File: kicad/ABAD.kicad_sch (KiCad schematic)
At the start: 5 parts, among them U1 MS5611-01BA, U2 ESP32-WROOM-32, U3 MPU-6050

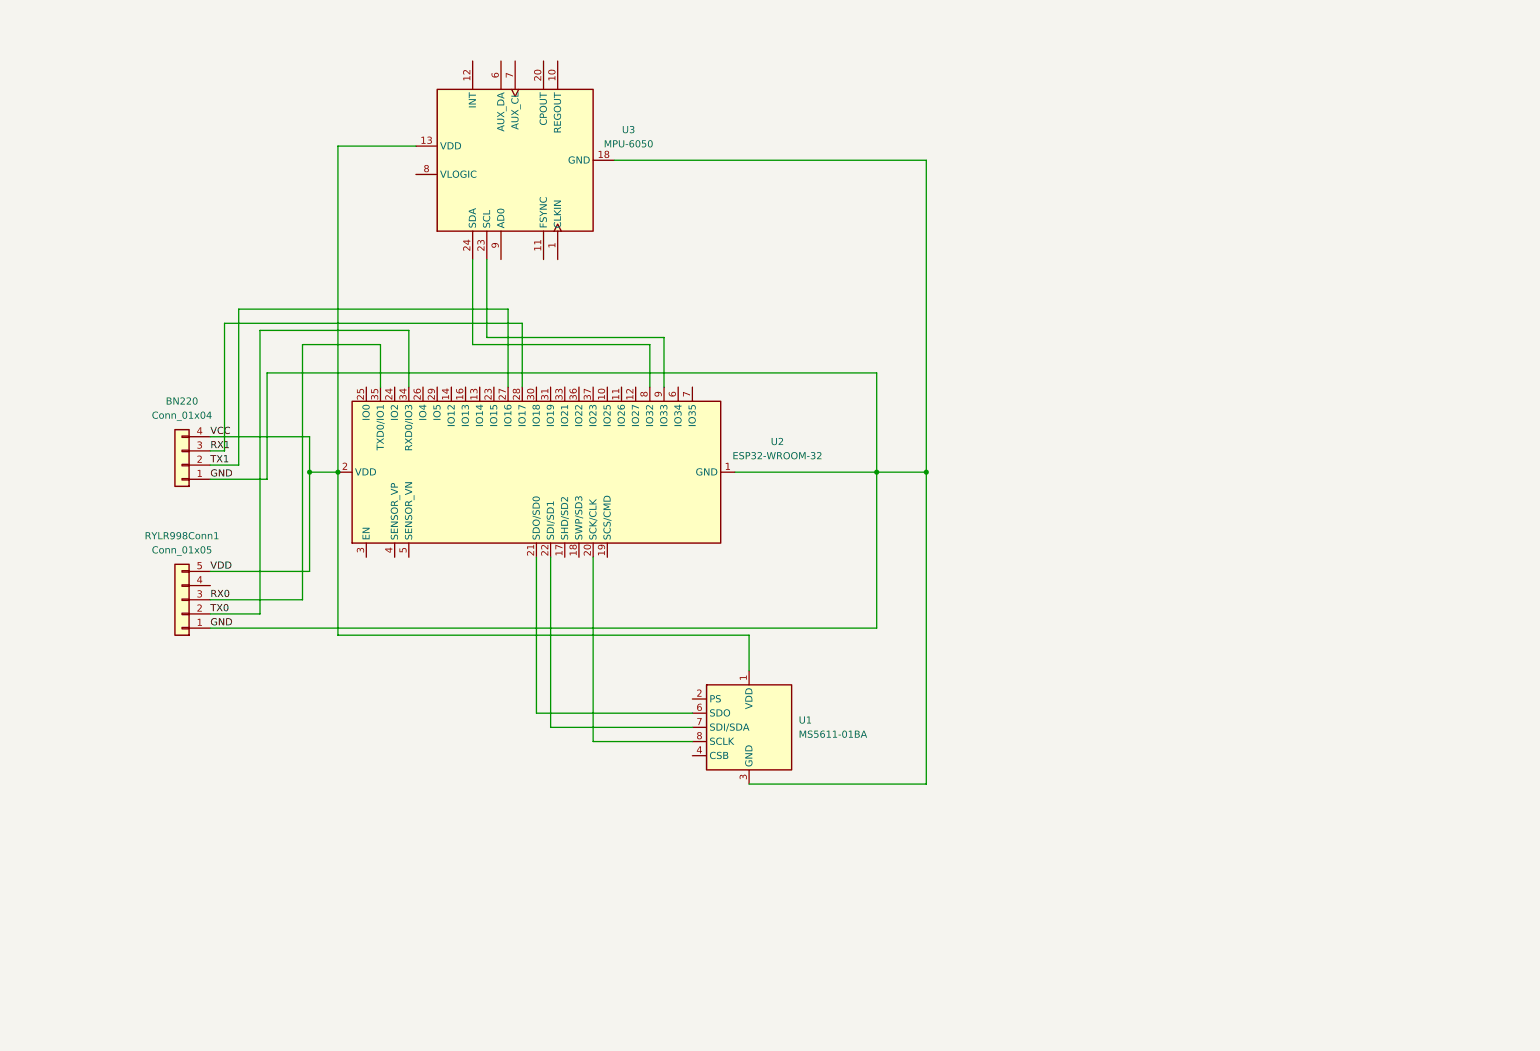
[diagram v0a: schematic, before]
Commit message: Schematic_Jul12_Nile
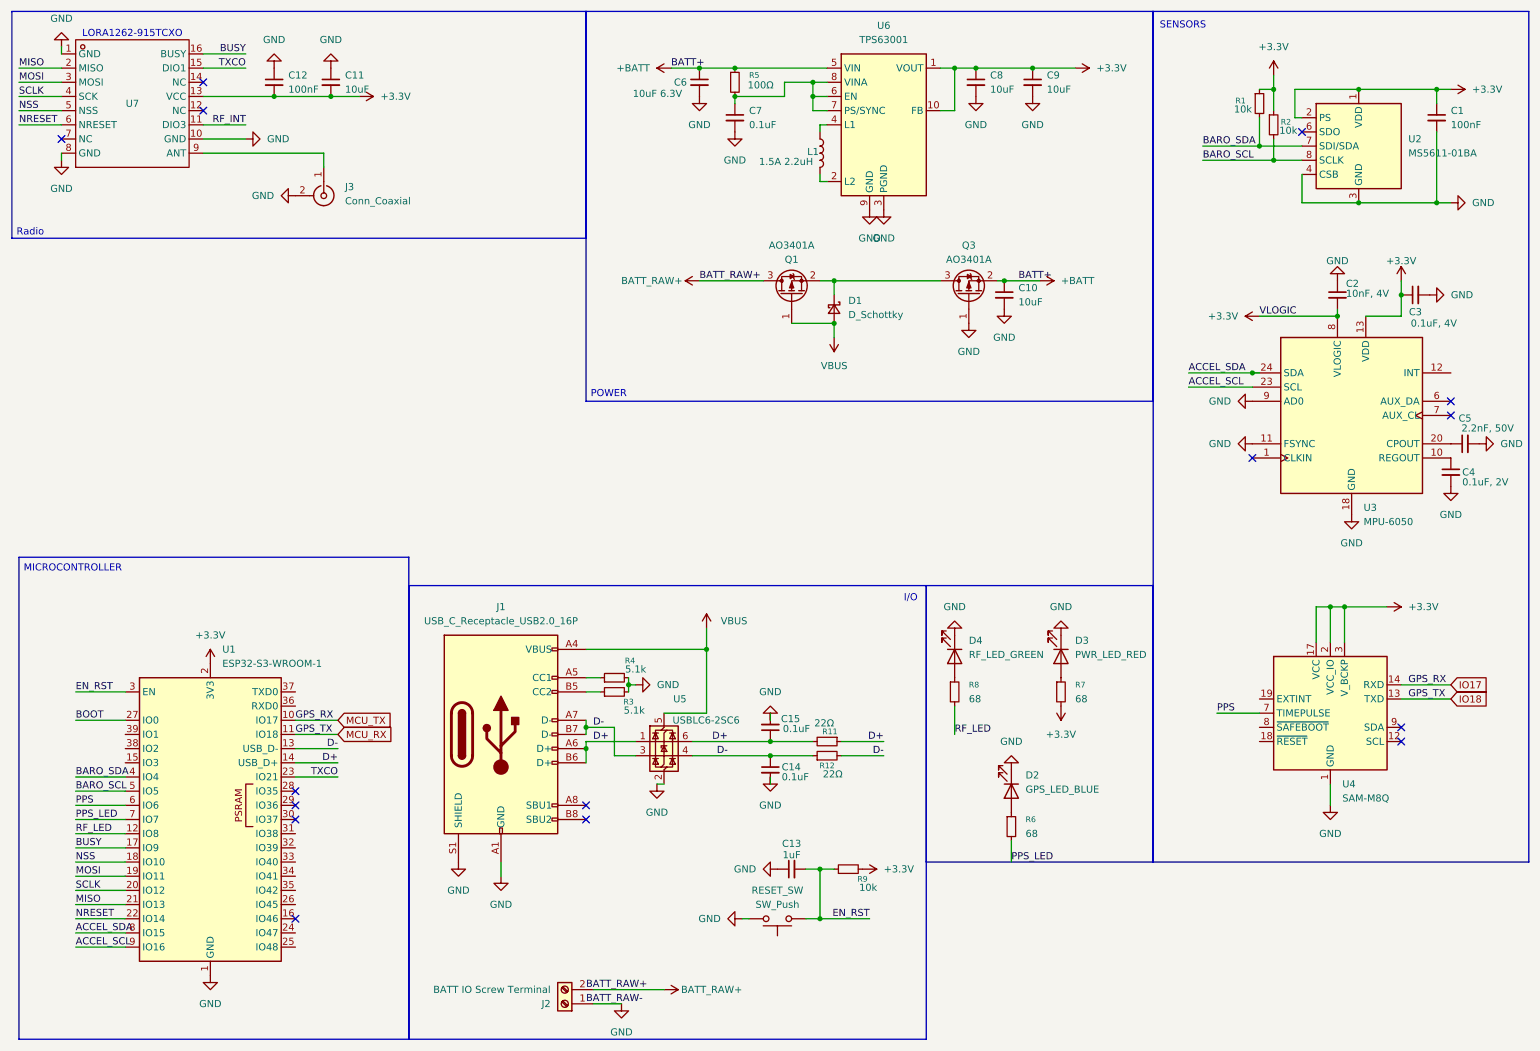
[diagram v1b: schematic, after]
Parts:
- removed BN220: Conn_01x04, Connector_JST:JST_SH_BM04B-SRSS-TB_1x04-1MP_P1.00mm_Vertical, symbol Connector_Generic:Conn_01x04
- removed RYLR998Conn1: Conn_01x05, Connector_PinSocket_1.00mm:PinSocket_1x05_P1.00mm_Vertical, symbol Connector_Generic:Conn_01x05
- removed U1: MS5611-01BA, Package_LGA:LGA-8_3x5mm_P1.25mm, symbol Sensor_Pressure:MS5611-01BA
- removed U2: ESP32-WROOM-32, RF_Module:ESP32-WROOM-32, symbol RF_Module:ESP32-WROOM-32
- added C1, C12: 100nF, Capacitor_SMD:C_0805_2012Metric, symbol Device:C_Small
- added C10, C11, C8, C9: 10uF, Capacitor_SMD:C_0805_2012Metric, symbol Device:C_Small
- added C13: 1uF, Capacitor_SMD:C_0805_2012Metric, symbol Device:C_Small
- added C14, C15, C7: 0.1uF, Capacitor_SMD:C_0805_2012Metric, symbol Device:C_Small
- added C2: 10nF, 4V, Capacitor_SMD:C_0805_2012Metric, symbol Device:C_Small
- added C3: 0.1uF, 4V, Capacitor_SMD:C_0805_2012Metric, symbol Device:C_Small
- added C4: 0.1uF, 2V, Capacitor_SMD:C_0805_2012Metric, symbol Device:C_Small
- added C5: 2.2nF, 50V, Capacitor_SMD:C_0805_2012Metric, symbol Device:C_Small
- added C6: 10uF 6.3V, Capacitor_SMD:C_0805_2012Metric, symbol Device:C_Small
- added D1: D_Schottky, Diode_SMD:D_3220_8050Metric, symbol Device:D_Schottky_Small
- added D2: GPS_LED_BLUE, LED_SMD:LED_0805_2012Metric, symbol Device:LED
- added D3: PWR_LED_RED, LED_SMD:LED_0805_2012Metric, symbol Device:LED
- added D4: RF_LED_GREEN, LED_SMD:LED_0805_2012Metric, symbol Device:LED
- added J1: USB_C_Receptacle_USB2.0_16P, Connector_USB:USB_Micro-B_Wuerth_629105150521_CircularHoles, symbol Connector:USB_C_Receptacle_USB2.0_16P
- added J2: BATT IO Screw Terminal, TerminalBlock_MetzConnect:TerminalBlock_MetzConnect_Type055_RT01502HDWU_1x02_P5.00mm_Horizontal, symbol Connector:Screw_Terminal_01x02
- added J3: Conn_Coaxial, Connector_Coaxial:SMA_Molex_73251-1153_EdgeMount_Horizontal, symbol Connector:Conn_Coaxial
- added L1: 1.5A 2.2uH, Inductor_SMD:L_0805_2012Metric, symbol Device:L
- added Q1, Q3: AO3401A, Package_TO_SOT_SMD:SOT-23, symbol Transistor_FET:AO3401A
- added R1, R2, R9: 10k, Resistor_SMD:R_0805_2012Metric, symbol Device:R_Small
- added R11, R12: 22Ω, Resistor_SMD:R_0805_2012Metric, symbol Device:R_Small
- added R3, R4: 5.1k, Resistor_SMD:R_0805_2012Metric, symbol Device:R_Small
- added R5: 100Ω, Resistor_SMD:R_0805_2012Metric, symbol Device:R_Small
- added R6, R7, R8: 68, Resistor_SMD:R_0805_2012Metric, symbol Device:R_Small
- added RESET_SW: SW_Push, symbol Switch:SW_Push
- added U1: ESP32-S3-WROOM-1, RF_Module:ESP32-S3-WROOM-1, symbol RF_Module:ESP32-S3-WROOM-1
- added U2: MS5611-01BA, Package_LGA:LGA-8_3x5mm_P1.25mm, symbol Sensor_Pressure:MS5611-01BA
- added U4: SAM-M8Q, RF_GPS:ublox_SAM-M8Q, symbol RF_GPS:SAM-M8Q
- added U5: USBLC6-2SC6, Package_TO_SOT_SMD:SOT-23-6, symbol Power_Protection:USBLC6-2SC6
- added U6: TPS63001, Package_SON:Texas_DRC0010J_ThermalVias, symbol Regulator_Switching:TPS63001
- added U7: ~, Lora1262_915TXCO:WIRELM-SMD_16P-L16.0-W16.0-P2.00_LORA-CC68-915MHZ-TCXO, symbol NiceRFLoRa1262_915:LORA1262-915TCXO
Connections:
- net VCC is gone; now on net +3.3V: U3.13 (VDD)
- net GND: now also U3.11 (FSYNC), U3.9 (AD0), C1.2, C10.2, C11.1, C12.1, C13.1, C14.2, C15.2, C2.1, C3.2, C4.2, C5.2, C6.2, C7.2, C8.2, C9.2, D2.1 (K), D3.1 (K), D4.1 (K), J1.A1 (GND), J1.A12 (GND), J1.B1 (GND), J1.B12 (GND), J1.S1 (SHIELD), J2.1 (Pin_1), J3.2 (Ext), Q3.1 (G), R3.2, R4.2, RESET_SW.2, U1.1 (GND), U1.40 (GND), U1.41 (GND), U2.3 (GND), U2.4 (CSB), U2.5 (CSB), U4.1 (GND), U4.10 (GND), U4.11 (GND), U4.15 (GND), U4.16 (GND), U4.20 (GND), U4.4 (GND), U4.5 (GND), U4.6 (GND), U5.2 (GND), U6.11 (PGND), U6.3 (PGND), U6.9 (GND), U7.1 (GND), U7.10 (GND), U7.8 (GND)
- net ACCEL_SDA: now reaches U3.24 (SDA)
- net ACCEL_SDA: now also U1.8 (IO15)
- net ACCEL_SCL: now reaches U3.23 (SCL)
- net ACCEL_SCL: now also U1.9 (IO16)
- net at U3.10 (REGOUT): now also C4.1
- net at U3.20 (CPOUT): now also C5.1
- net +3.3V: now reaches U3.8 (VLOGIC)
- net +3.3V: now also C1.1, C11.2, C12.2, C2.2, C3.1, C8.1, C9.1, R1.1, R2.1, R7.2, R9.2, U1.2 (3V3), U2.1 (VDD), U2.2 (PS), U4.17 (VCC), U4.2 (VCC_IO), U4.3 (V_BCKP), U6.1 (VOUT), U6.10 (FB), U7.13 (VCC)
- new net: J1.A5 (CC1), R4.1
- new net: D3.2 (A), R7.1
- new net: C7.1, R5.2, U6.6 (EN), U6.7 (PS/SYNC), U6.8 (VINA)
- new net: J3.1 (In), U7.9 (ANT)
- new net: L1.1, U6.4 (L1)
- new net: L1.2, U6.2 (L2)
- new net: D1.1 (K), Q1.2 (S), Q3.3 (D)
- new net: D2.2 (A), R6.1
- new net: J1.B5 (CC2), R3.1
- new net: D4.2 (A), R8.1
- new net +BATT: C10.1, C6.1, Q3.2 (S), R5.1, U6.5 (VIN)
- new net BARO_SCL: R2.2, U1.5 (IO5), U2.8 (SCLK)
- new net BARO_SDA: R1.2, U1.4 (IO4), U2.7 (SDI/SDA)
- new net BATT_RAW+: J2.2 (Pin_2), Q1.3 (D)
- new net BOOT: U1.27 (IO0)
- new net BUSY: U1.17 (IO9), U7.16 (BUSY)
- new net D+: C15.1, J1.A6 (D+), J1.B6 (D+), R11.1, R11.2, U1.14 (USB_D+), U5.1 (I/O1), U5.6 (I/O1)
- new net D-: C14.1, J1.A7 (D-), J1.B7 (D-), R12.1, R12.2, U1.13 (USB_D-), U5.3 (I/O2), U5.4 (I/O2)
- new net EN_RST: C13.2, R9.1, RESET_SW.1, U1.3 (EN)
- new net IO17: U1.10 (IO17), U4.14 (RXD)
- new net IO18: U1.11 (IO18), U4.13 (TXD)
- new net MISO: U1.21 (IO13), U7.2 (MISO)
- new net MOSI: U1.19 (IO11), U7.3 (MOSI)
- new net NRESET: U1.22 (IO14), U7.6 (NRESET)
- new net NSS: U1.18 (IO10), U7.5 (NSS)
- new net PPS: U1.6 (IO6), U4.7 (TIMEPULSE)
- new net PPS_LED: R6.2, U1.7 (IO7)
- new net RF_INT: U7.11 (DIO3)
- new net RF_LED: R8.2, U1.12 (IO8)
- new net SCLK: U1.20 (IO12), U7.4 (SCK)
- new net TXCO: U1.23 (IO21), U7.15 (DIO1)
- new net VBUS: D1.2 (A), J1.A4 (VBUS), J1.A9 (VBUS), J1.B4 (VBUS), J1.B9 (VBUS), Q1.1 (G), U5.5 (VBUS)
- no-connect marks 0 -> 15
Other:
- note added: "I/O"
- note added: "LORA1262-915TCXO"
- note added: "MICROCONTROLLER"
- note added: "POWER"
- note added: "Radio"
- note added: "SENSORS"
